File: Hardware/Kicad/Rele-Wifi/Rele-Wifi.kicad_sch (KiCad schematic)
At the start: 46 parts, among them J13 Screw_Terminal, SW1 SW_DPST_x2, U1 817C, U2 817C, U3 817C, U4 817C, U5 L7805, U7 ESP32_DevKit_V1_CH9102X

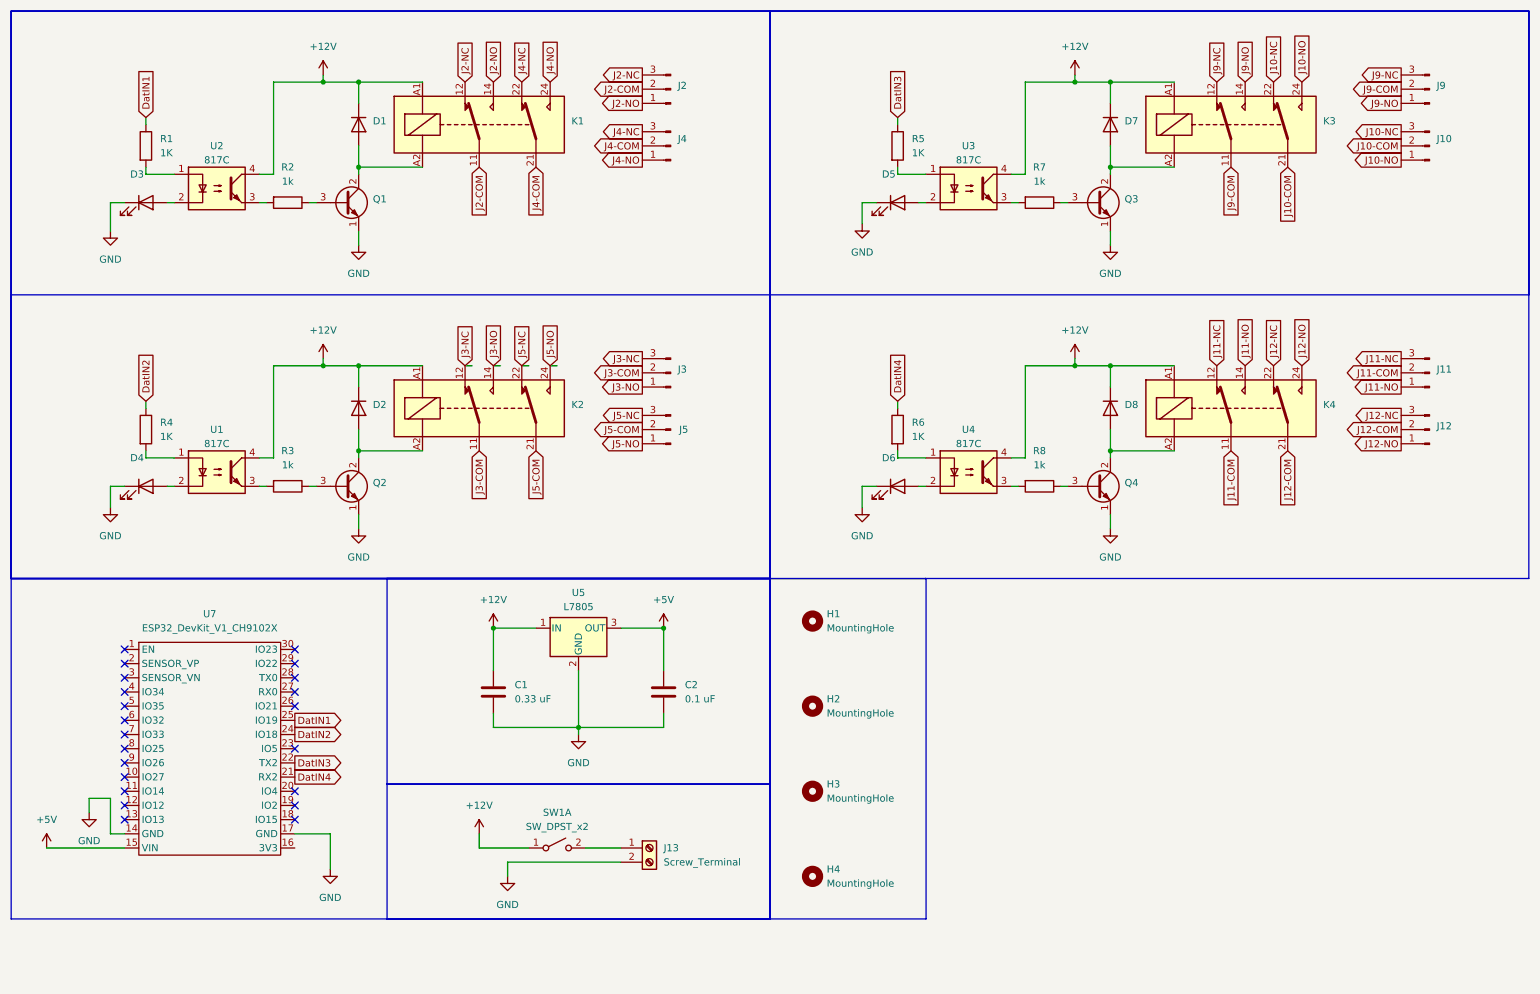
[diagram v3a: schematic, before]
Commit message: Ultima Revision
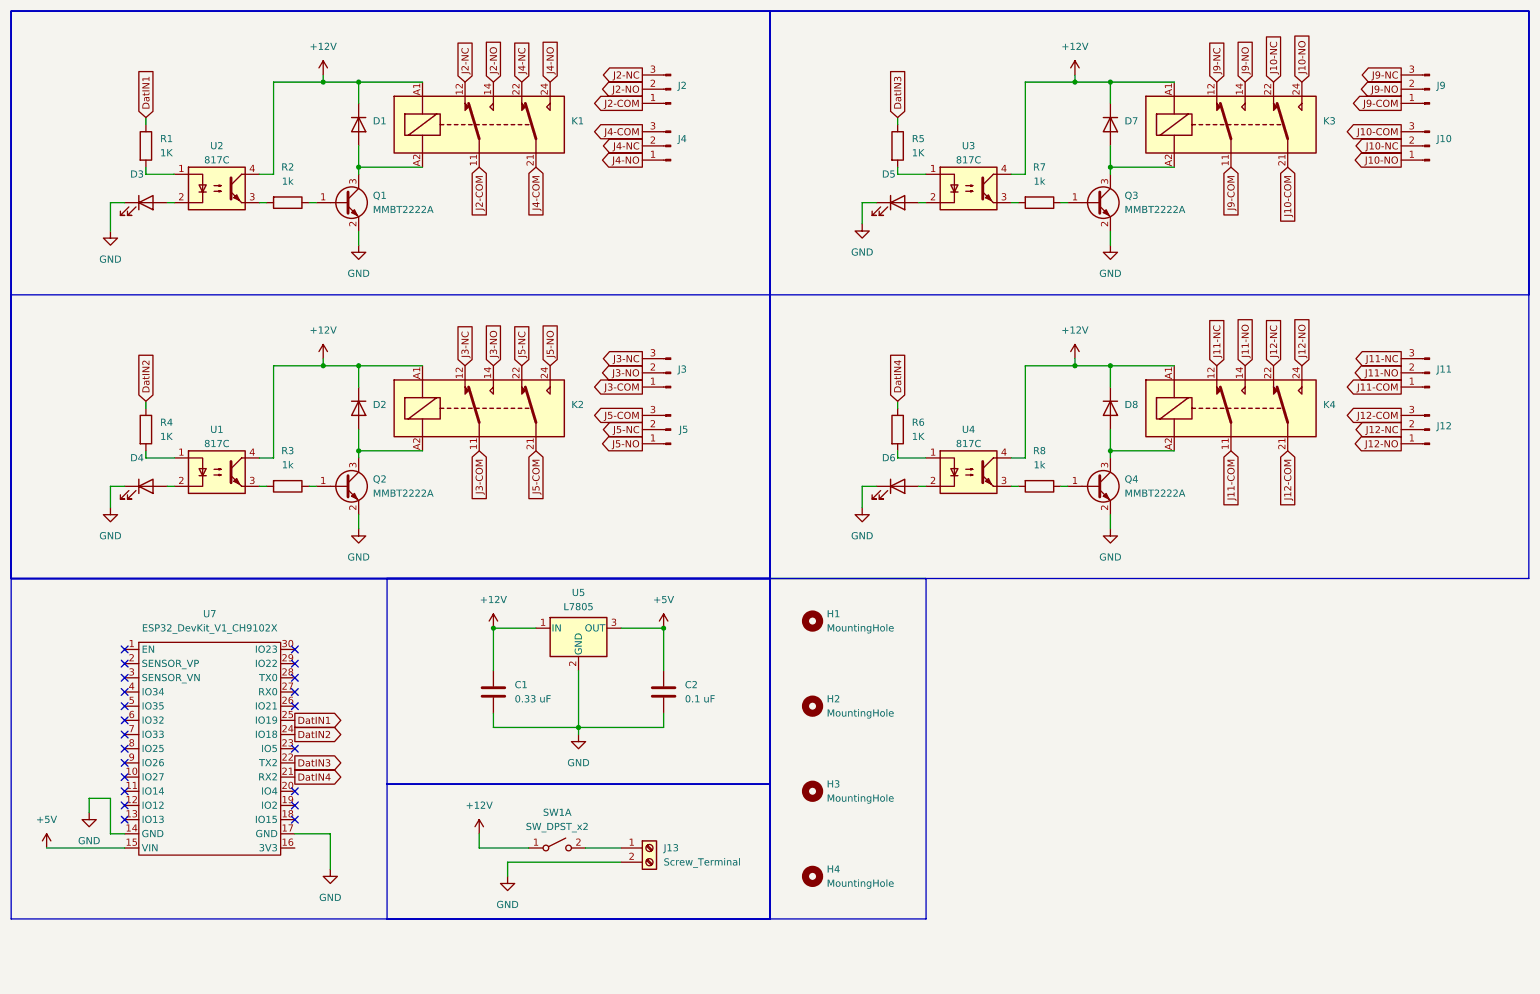
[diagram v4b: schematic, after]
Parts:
- removed Q1, Q2, Q3, Q4: ~, Package_TO_SOT_SMD:SOT-23, symbol Transistor_BJT:BF457
- added Q1, Q2, Q3, Q4: MMBT2222A, Package_TO_SOT_SMD:SOT-23, symbol Transistor_BJT:MMBT2222A
- D1, D2, D7, D8: footprint Diode_SMD:D_0805_2012Metric -> Diode_SMD:D_SMA
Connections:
- net GND: now also Q1.2 (E), Q2.2 (E), Q3.2 (E), Q4.2 (E)
- net J10-COM: now also J10.3 (Pin_3); no longer J10.2 (Pin_2)
- net J10-NC: now also J10.2 (Pin_2); no longer J10.3 (Pin_3)
- net J11-COM: now also J11.1 (Pin_1); no longer J11.2 (Pin_2)
- net J11-NO: now also J11.2 (Pin_2); no longer J11.1 (Pin_1)
- net J12-COM: now also J12.3 (Pin_3); no longer J12.2 (Pin_2)
- net J12-NC: now also J12.2 (Pin_2); no longer J12.3 (Pin_3)
- net J2-COM: now also J2.1 (Pin_1); no longer J2.2 (Pin_2)
- net J2-NO: now also J2.2 (Pin_2); no longer J2.1 (Pin_1)
- net J3-COM: now also J3.1 (Pin_1); no longer J3.2 (Pin_2)
- net J3-NO: now also J3.2 (Pin_2); no longer J3.1 (Pin_1)
- net J4-COM: now also J4.3 (Pin_3); no longer J4.2 (Pin_2)
- net J4-NC: now also J4.2 (Pin_2); no longer J4.3 (Pin_3)
- net J5-COM: now also J5.3 (Pin_3); no longer J5.2 (Pin_2)
- net J5-NC: now also J5.2 (Pin_2); no longer J5.3 (Pin_3)
- net J9-COM: now also J9.1 (Pin_1); no longer J9.2 (Pin_2)
- net J9-NO: now also J9.2 (Pin_2); no longer J9.1 (Pin_1)
- net at D7.2 (A), K3.A2: now also Q3.3 (C)
- net at R7.1: now also Q3.1 (B)
- net at D1.2 (A), K1.A2: now also Q1.3 (C)
- net at R8.1: now also Q4.1 (B)
- net at R2.1: now also Q1.1 (B)
- net at D8.2 (A), K4.A2: now also Q4.3 (C)
- net at R3.1: now also Q2.1 (B)
- net at D2.2 (A), K2.A2: now also Q2.3 (C)
